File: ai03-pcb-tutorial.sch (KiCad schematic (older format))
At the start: 5 parts

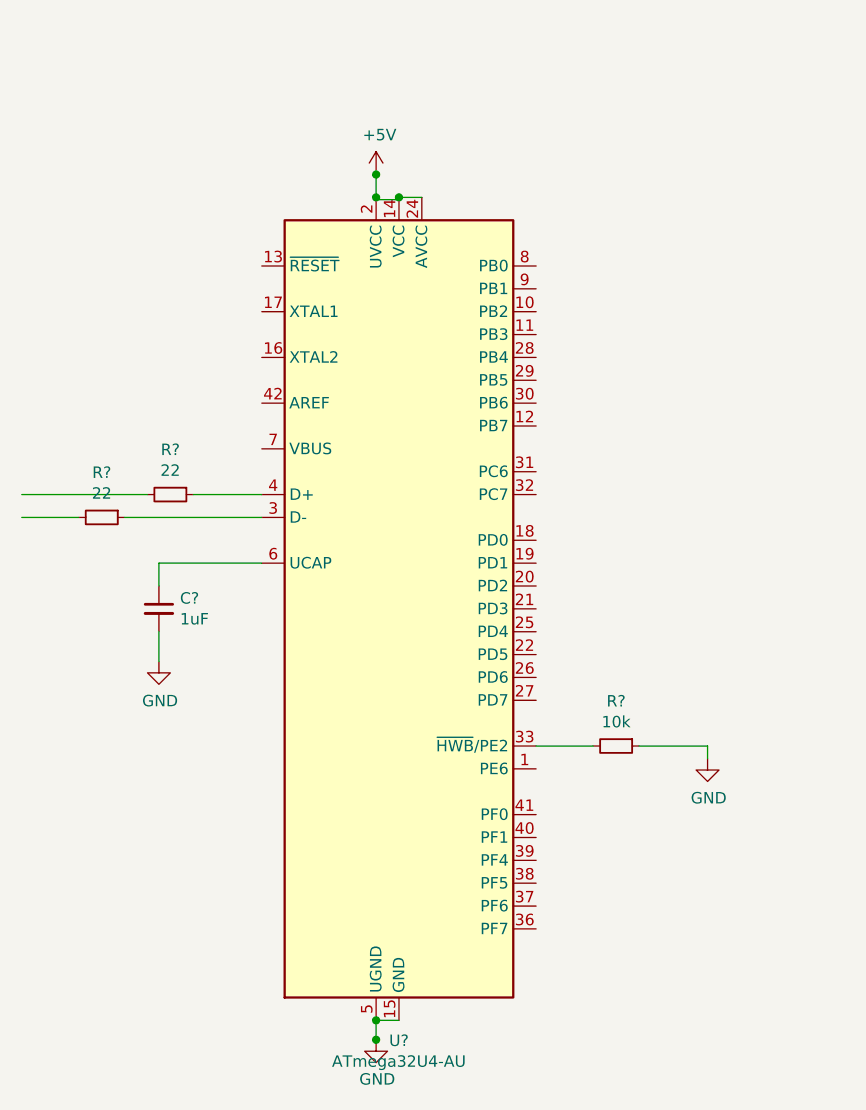
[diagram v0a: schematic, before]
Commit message: set reset switch, crystal
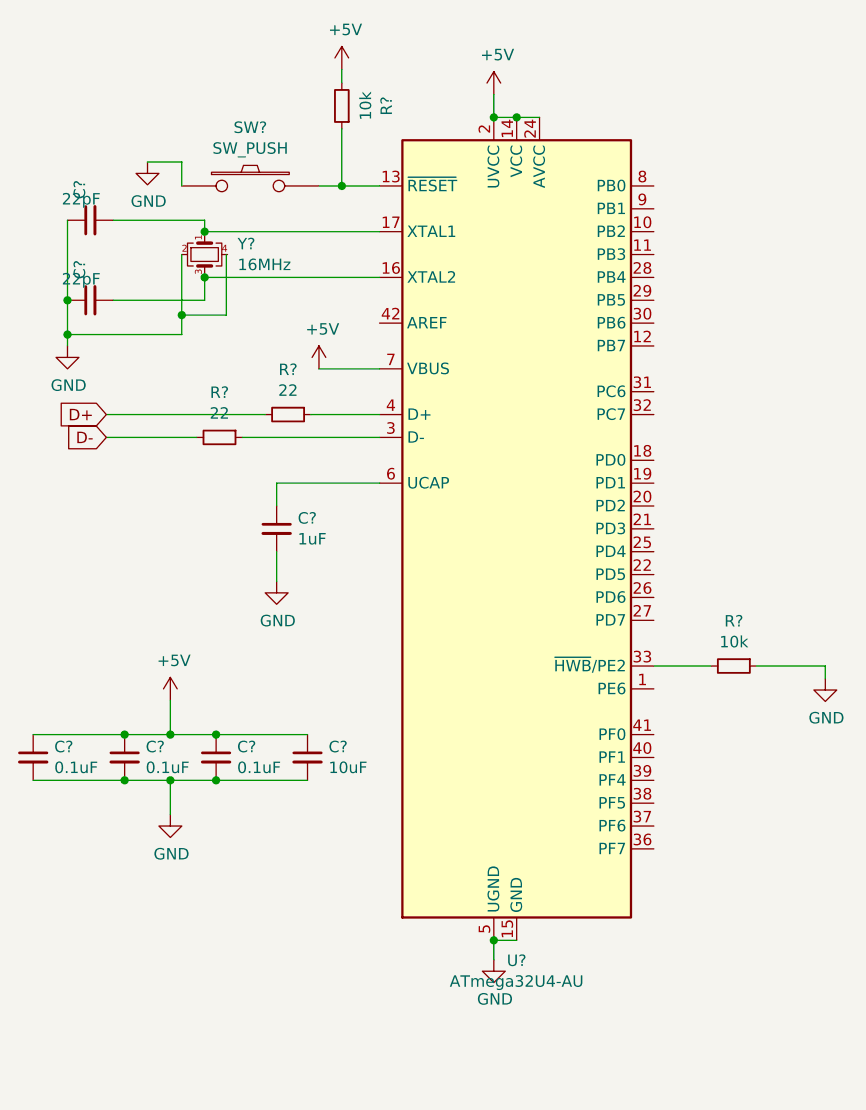
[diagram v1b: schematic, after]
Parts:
- added C? (x3): 0.1uF, symbol Device:C_Small
- added C?: 10uF, symbol Device:C_Small
- added C? (x2): 22pF, symbol Device:C_Small
- added R?: 10k, symbol Device:R_Small
- added SW?: SW_PUSH, symbol kbd:SW_PUSH
- added Y?: 16MHz, symbol Device:Crystal_GND24_Small
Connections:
- net labels added: D+, D-
- wire segments 20 -> 46
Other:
- moved on the sheet: C?, R?, U?
